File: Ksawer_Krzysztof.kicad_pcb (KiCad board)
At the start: 2 copper layers, 57 parts, among them J1 BAT, J3 V1, K1 1461103-1, K2 1461103-1, Q1 BC547, Q2 MMBT3904, Q3 MMBT3904, U1 DHT11, U2 ESP-12E, U3 NHD-C0220BIZ, U4 LTV-844, U5 STM32F038K6Ux, U6 TPS63021DSJR, U8 INA180A1, Y1 ABM3-B.000MHZ-D2Y

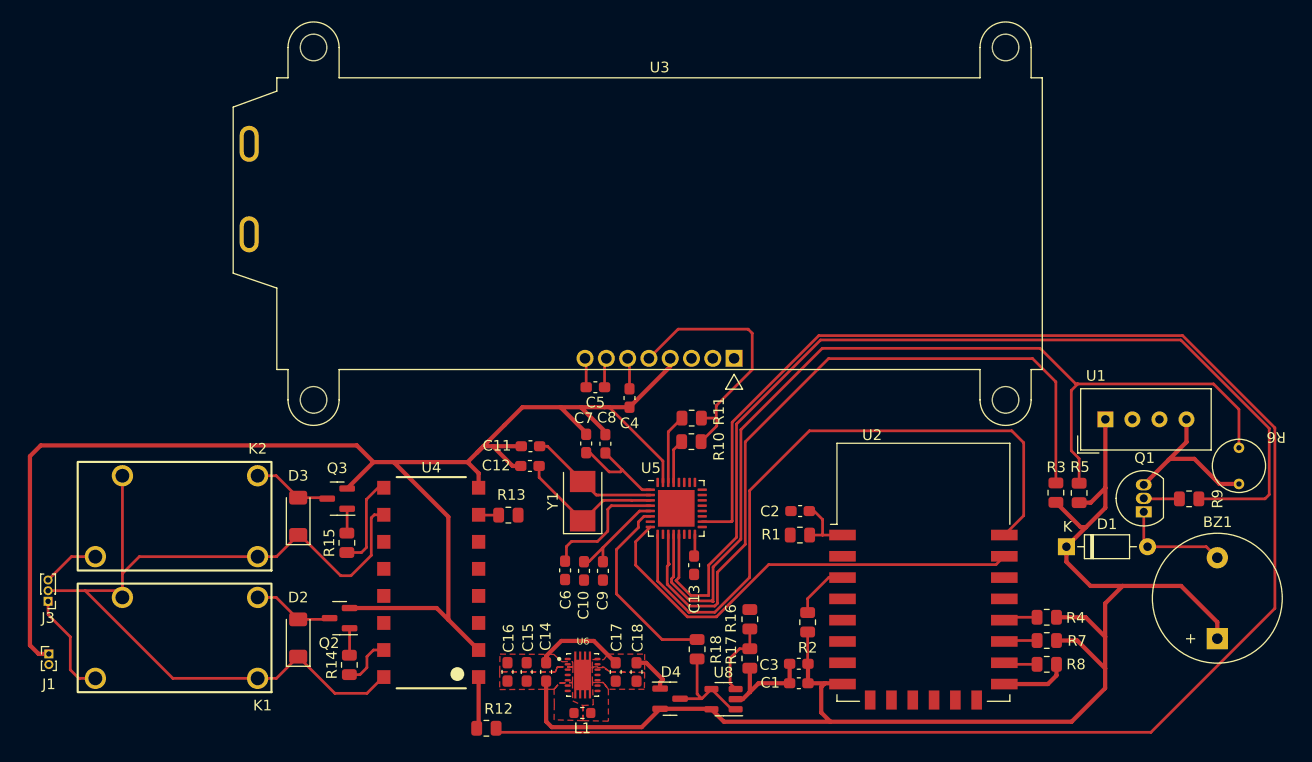
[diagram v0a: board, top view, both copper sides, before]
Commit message: prawie koniec
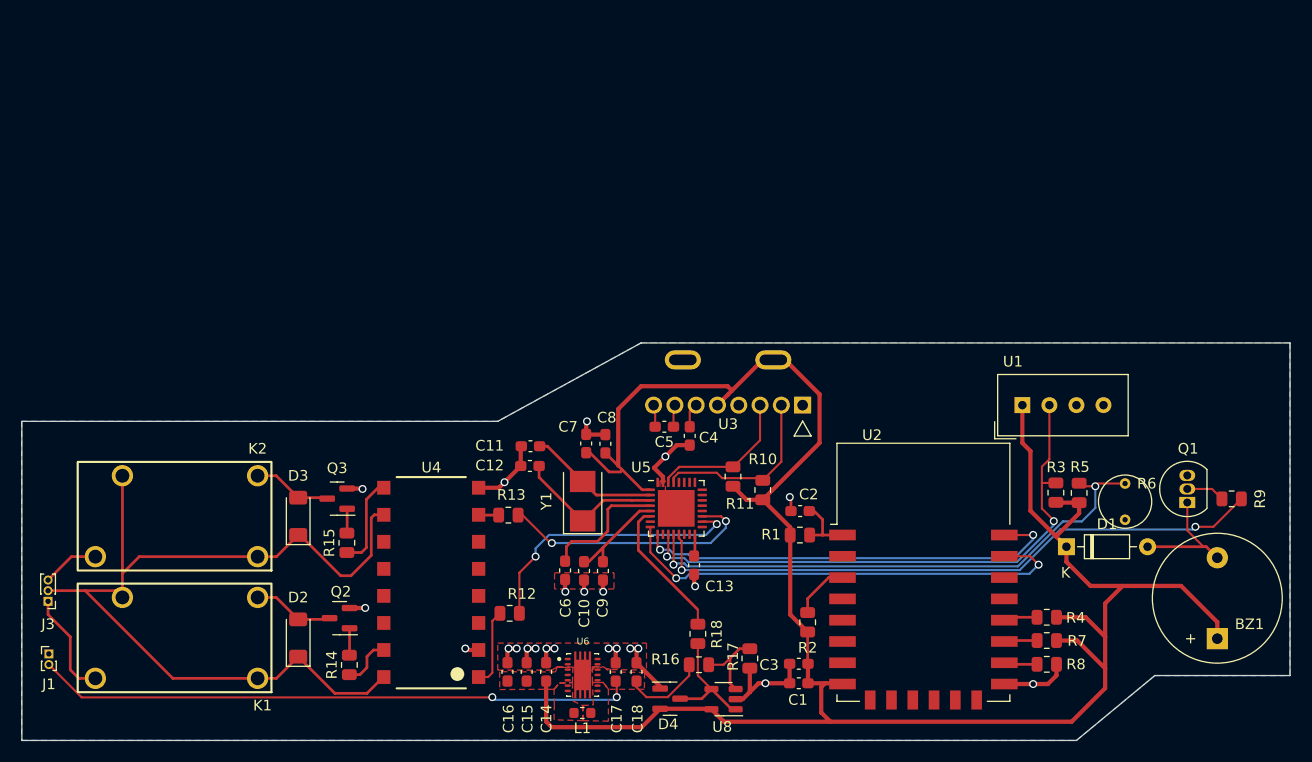
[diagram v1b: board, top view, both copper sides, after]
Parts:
- U3: footprint Display:NHD-C0220BiZ -> Trans_footprint:NHD-C0220BiZ
- moved U3 21.3 mm to (154.0, 93.5)
- moved R6 11.2 mm to (191.3, 100.8)
- moved R12 11.0 mm to (133.5, 113.0)
- moved R10 8.10 mm to (157.2, 101.4), turned to 90 degrees
- moved U1 7.91 mm to (181.6, 93.5)
- moved C5 7.47 mm to (148.0, 95.5)
- moved R11 6.72 mm to (154.4, 100.2), turned to 90 degrees
- moved C4 6.69 mm to (150.4, 96.4)
- moved R16 6.41 mm to (151.2, 117.9), turned to 0 degrees
- moved Q1 4.18 mm to (197.1, 102.6)
- moved R9 4.00 mm to (201.3, 102.3)
- moved R18 1.45 mm to (151.1, 115.0)
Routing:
- net Data4: track 165.1 -> 26.2 mm, vias 0 -> 2
- net GND: track 190.8 -> 57.6 mm, vias 0 -> 23
- net +BATT: track 0.00 -> 64.2 mm, vias 0 -> 2
- net Data2: track 92.3 -> 51.5 mm, vias 0 -> 2
- net VDD: track 166.8 -> 204.5 mm
- net Data3: track 95.1 -> 58.8 mm, vias 0 -> 2
- net Data5: track 0.00 -> 24.2 mm, vias 0 -> 2
- net USART1_RX: track 61.7 -> 40.8 mm, vias 0 -> 2
- net Data1: track 69.6 -> 53.5 mm, vias 0 -> 2
- net SCL: track 4.56 -> 17.1 mm
- net SDA: track 6.69 -> 13.8 mm
- net /VBAT_ADC: track 18.3 -> 13.3 mm
- net Net-(R12-Pad2): track 4.89 -> 7.34 mm
- net Net-(BZ1-+): track 10.4 -> 12.3 mm
- net Net-(D4-COM): track 10.7 -> 11.6 mm
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- added copper zone on B.Cu, net GND
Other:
- board outline added: 119.1 x 37.3 mm
